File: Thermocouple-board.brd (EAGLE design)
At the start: 76.2 x 76.2 mm, 75 parts, among them J1 RJ45, J11 1X2-3.5MM, J12 1X2-3.5MM, J13 1X2-3.5MM, J14 1X2-3.5MM, J2 RJ45, J3 1981584-1, SW1 PUSHBUTTON, SW2 PUSHBUTTON, U1 STM32F042K4, U10 MAX31855, U11 MAX31855, U12 MAX31855, U13 MAX31855, U20 EEPROM-I2C, U21 EEPROM-I2C, U30 ST3485, U31 ST3485, U40 LP298XS, X1 NX3225GD

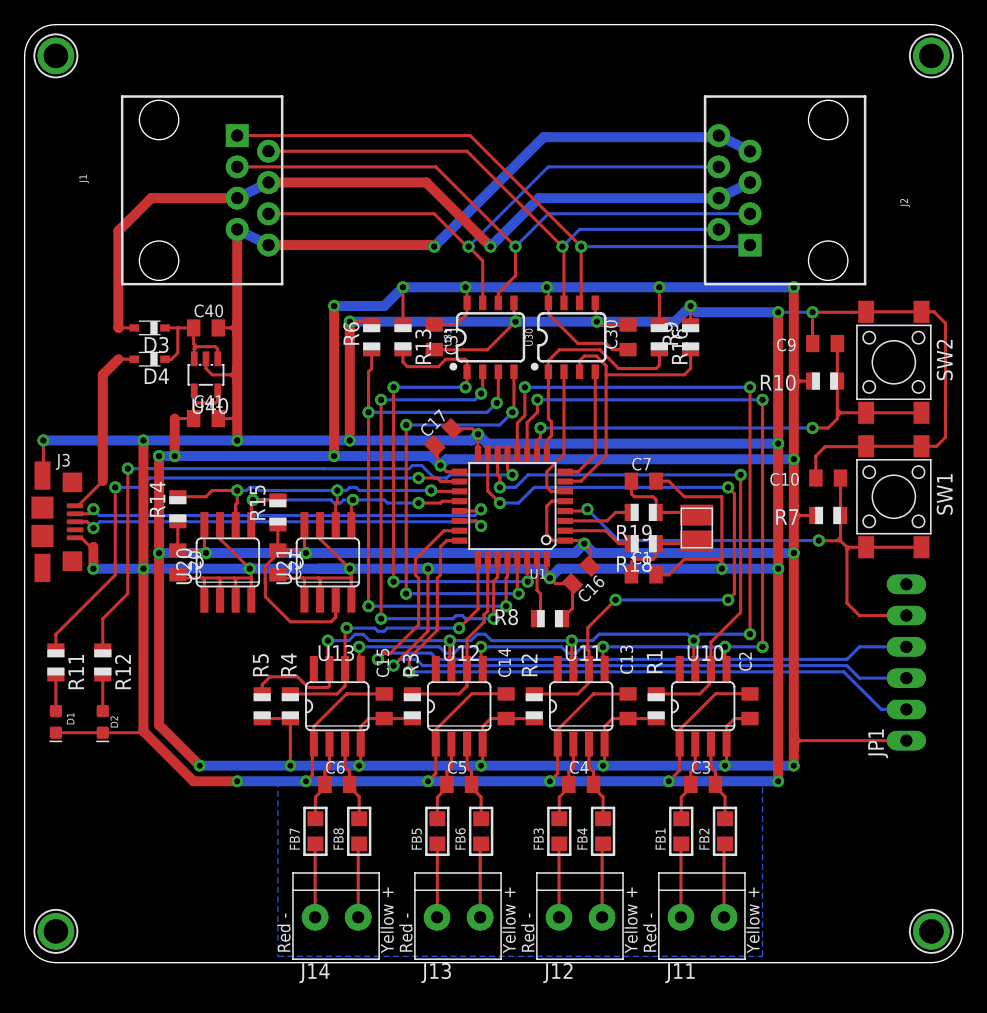
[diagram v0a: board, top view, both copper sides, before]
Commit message: First pass routing commplete
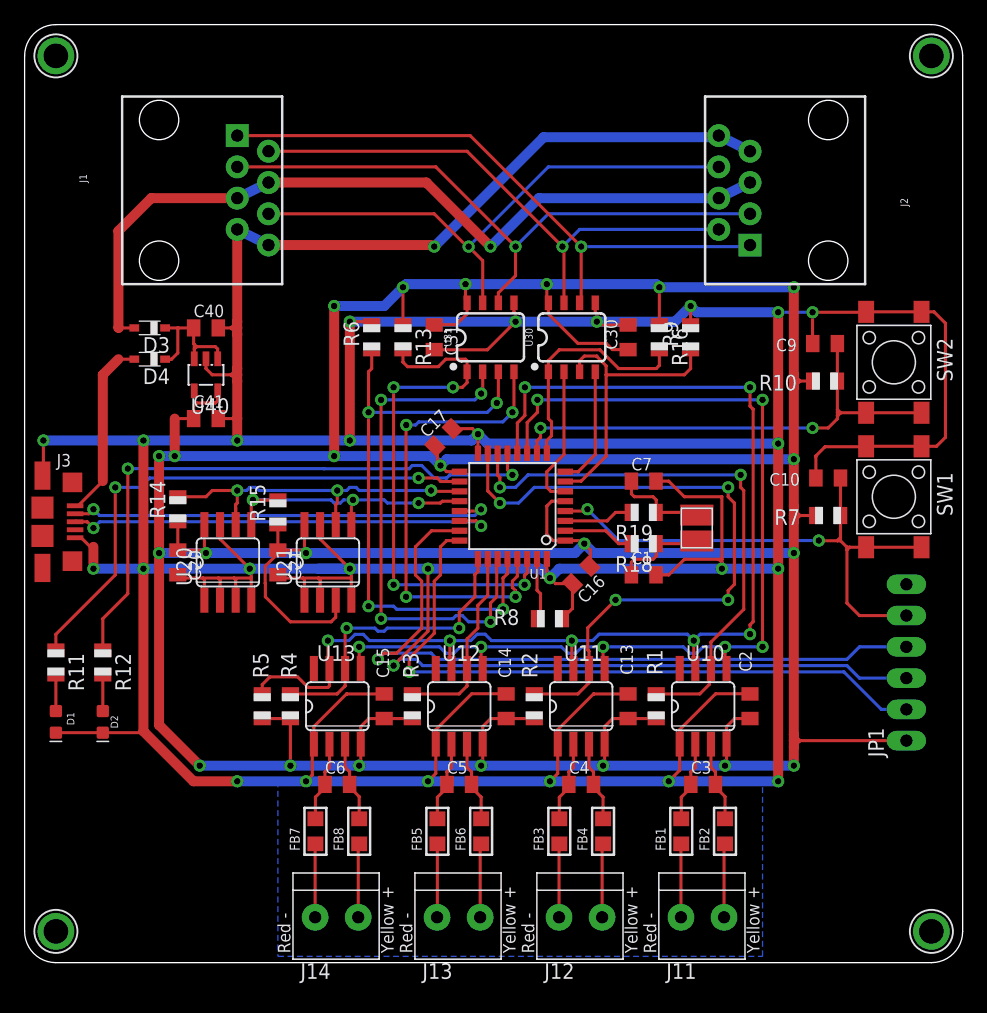
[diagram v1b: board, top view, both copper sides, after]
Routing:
- net SWDIO: track 58.3 -> 59.4 mm
- net +3V3: track 389.5 -> 390.2 mm
- net UART1_RX: track 43.5 -> 44.0 mm
